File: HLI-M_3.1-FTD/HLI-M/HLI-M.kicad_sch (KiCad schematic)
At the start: 116 parts, among them CON1 , CON2 USB_B, CON3 , CON4 Connector_Adapter, CON5 Connector_Audio, CON6 Conn_01x15, CON7 Conn_01x09, CON8 CR123A, Q1 DMP3068L-7, Q2 BC817, Q3 BC817, Q4 BSS84, Q5 BSS84, Q6 BSS84, Q7 BSS84, U1 PIC24HJ64GP206-I_PT, U10 24AA02-OT, U11 ULN2003, U12 ULN2003, U13 ULN2003, U2 FM25V10-GTR, U3 MAX3232, U4 TPS7A0533PDBV, U5 TPS7A0533PDBV, U6 LM3658SD, U8 FT232RL, U9 ATSHA204A-SSHDA-B, Y1 Crystal_32KHz, Y2 Crystal_20MHz

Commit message: att
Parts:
- removed CON5: Connector_Audio, Connector_JST:JST_EH_B3B-EH-A_1x03_P2.50mm_Vertical, symbol Connector_Generic:Conn_01x03
- removed RT3: 0.5A, Resistor_SMD:R_1812_4532Metric, symbol Device:Thermistor
- added CON5: Connector_note, Connector_IDC:IDC-Header_2x04_P2.54mm_Horizontal, symbol Connector_Generic:Conn_02x04_Odd_Even
- added F1: Fuse, Fuse:Fuse_1812_4532Metric, symbol Device:Fuse
- added RV1: Varistor, Capacitor_SMD:C_0603_1608Metric_Pad1.08x0.95mm_HandSolder, symbol Device:Varistor
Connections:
- net +5V: now also CON5.1 (Pin_1), F1.2, RV1.2
- net 0: now also CON5.8 (Pin_8), RV1.1
- net INIB: now also CON5.2 (Pin_2)
- net NOTE_: now also CON5.4 (Pin_4)
- net PRINT_IMP: now also CON5.6 (Pin_6)
- net RXA: now also CON5.3 (Pin_3)
- net TXA: now also CON5.5 (Pin_5)
- net at CON1.1 (Pin_1): now also F1.1
- net EXTERN_D10: now reaches U1.44 (RD10)
- net EXTERN_D10: now also CON5.7 (Pin_7)
- no-connect marks 36 -> 35
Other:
- moved on the sheet: CON1, CON4, LED2, LED3, R25, R26, R27, R28, TP1, TP2, TP3, TP4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

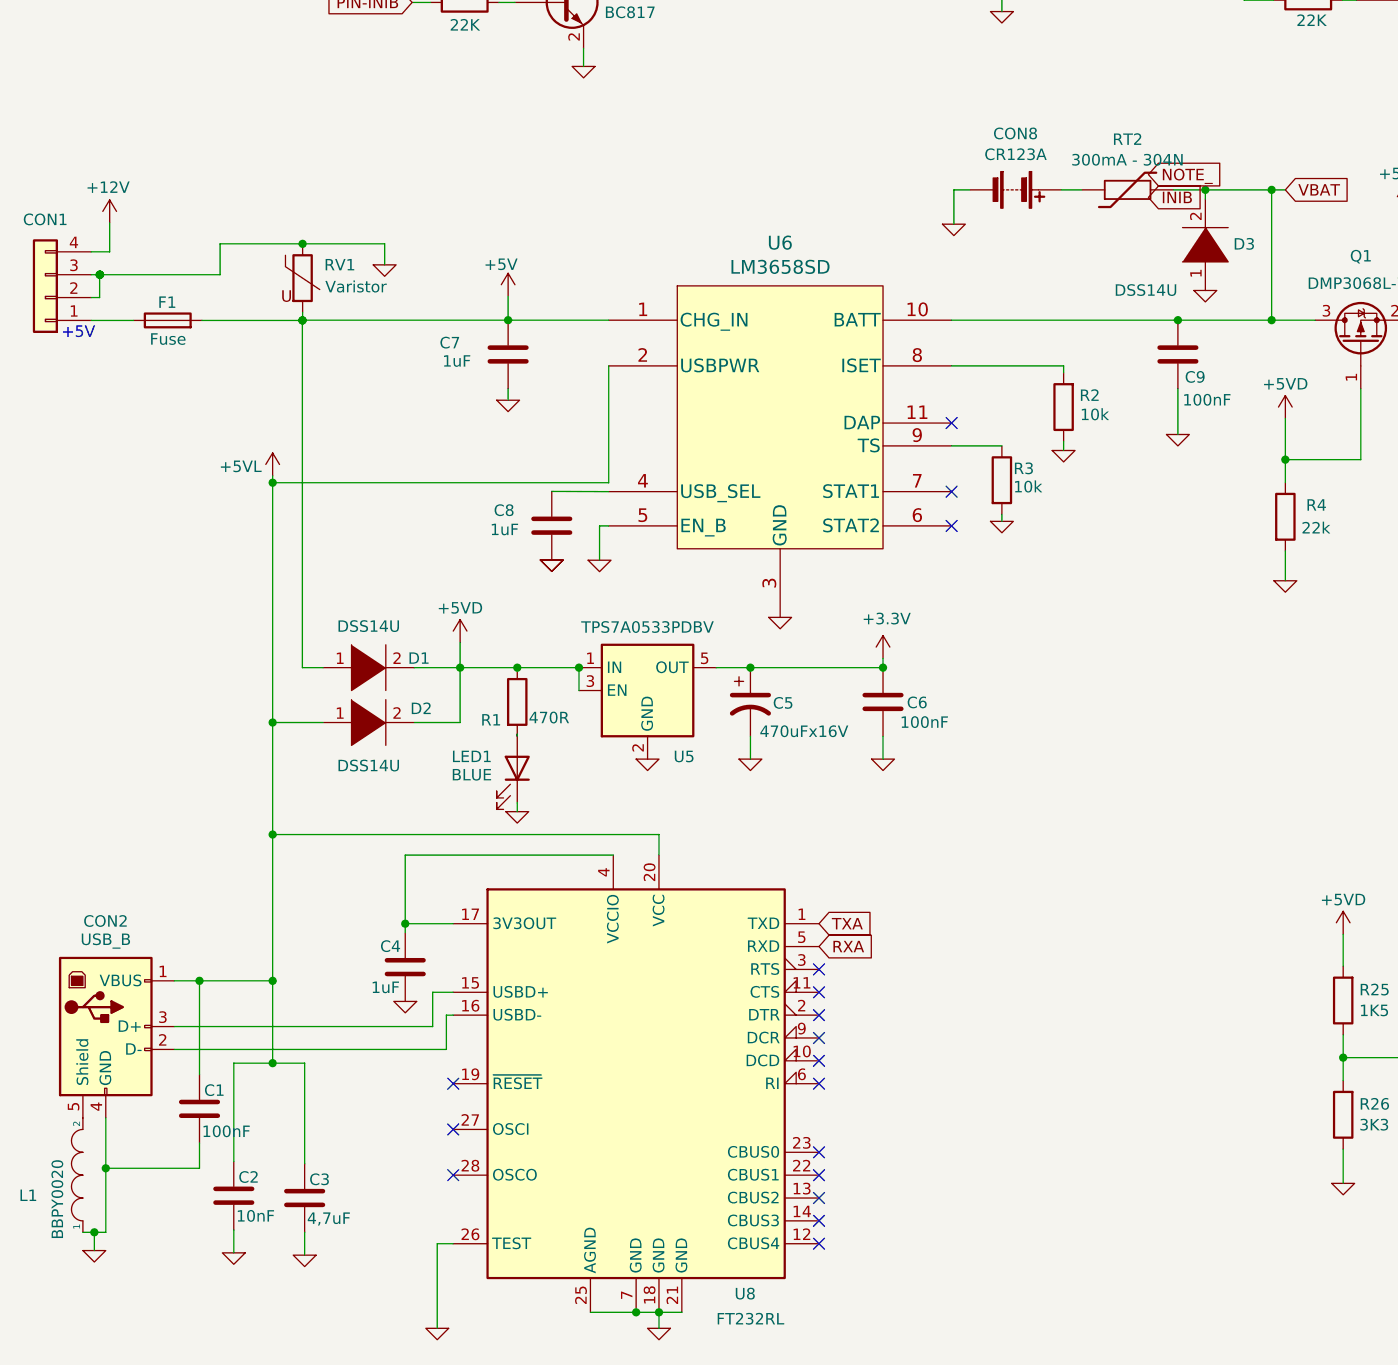
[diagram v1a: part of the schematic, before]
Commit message: att
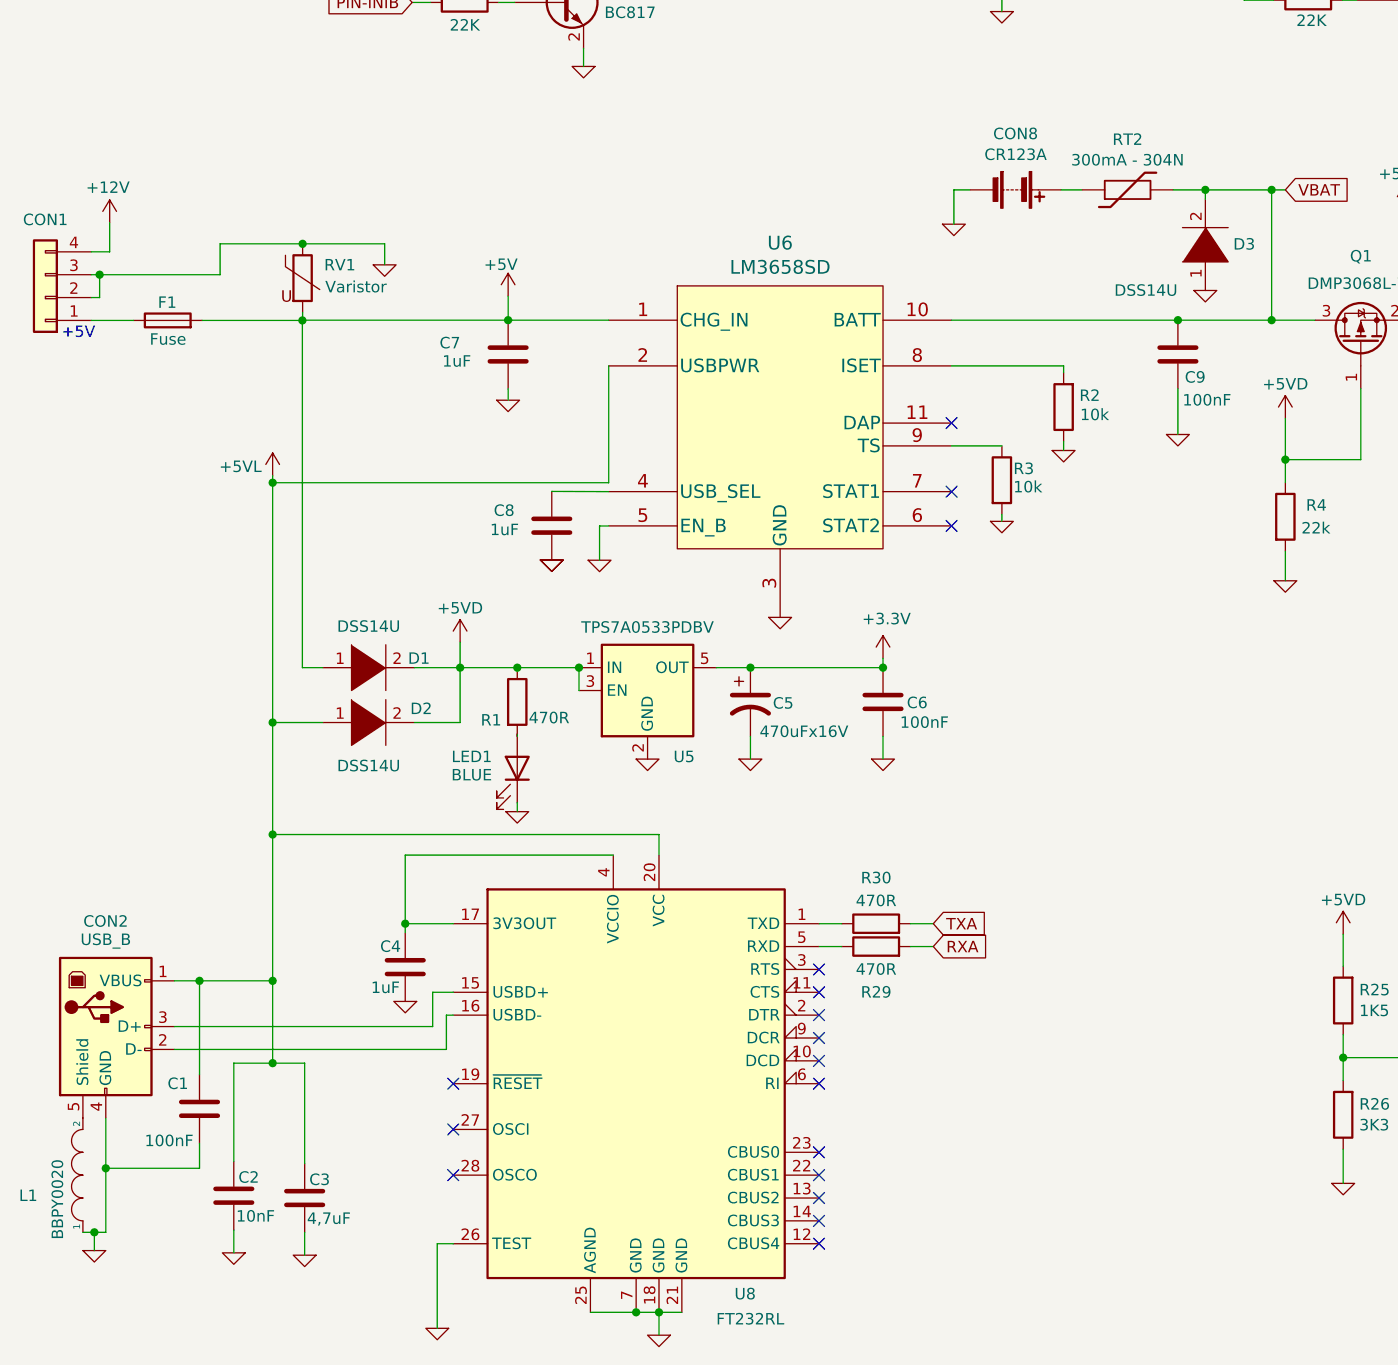
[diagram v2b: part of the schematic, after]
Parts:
- added R29, R30: 470R, symbol Device:R
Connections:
- net RXA: now also R29.2; no longer U8.5 (RXD)
- net TXA: now also R30.2; no longer U8.1 (TXD)
- new net: R29.1, U8.5 (RXD)
- new net: R30.1, U8.1 (TXD)

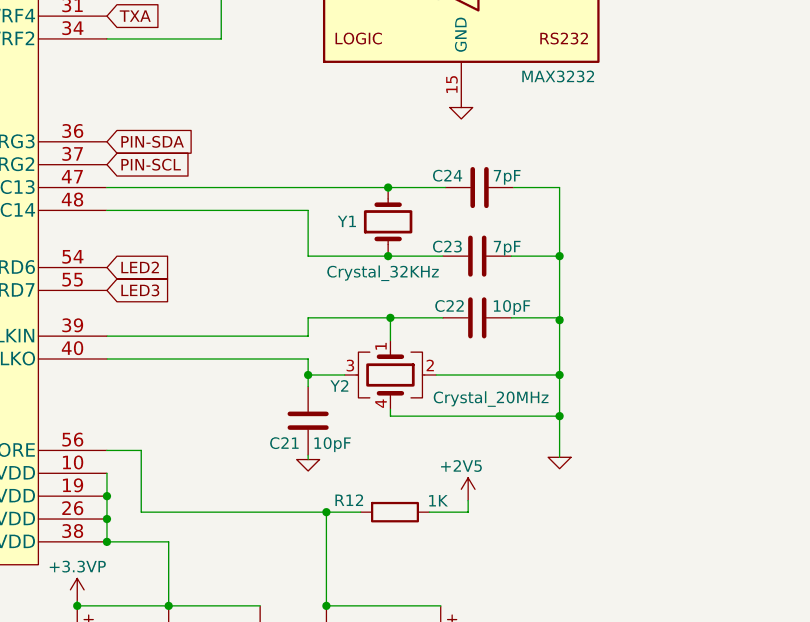
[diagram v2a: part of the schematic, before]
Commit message: atualização circuito FTD e 3D
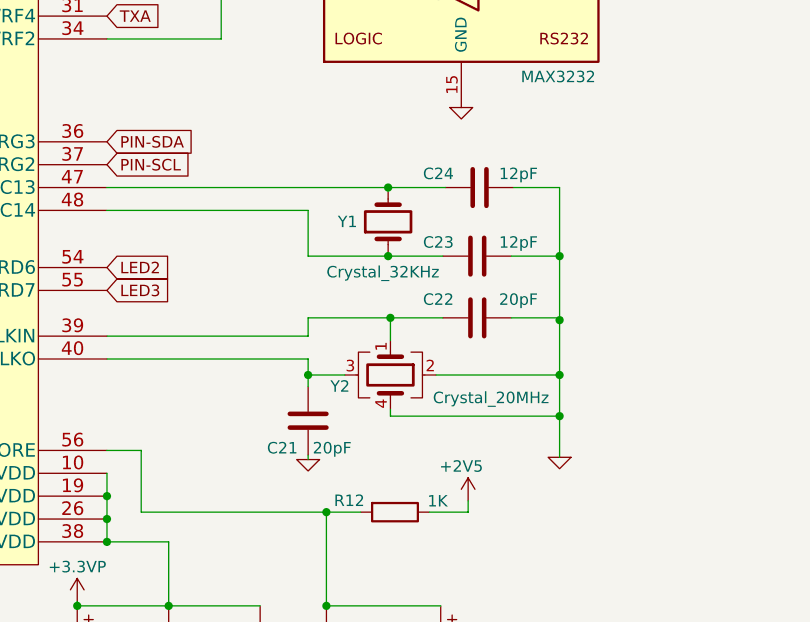
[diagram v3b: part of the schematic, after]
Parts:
- C21, C22: value 10pF -> 20pF
- C23, C24: value 7pF -> 12pF
- R29, R30: footprint (none) -> Resistor_SMD:R_0603_1608Metric_Pad0.98x0.95mm_HandSolder
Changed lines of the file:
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@@
       (effects (font (size 1.27 1.27)))
     )
-    (property "Footprint" "" (at 110.49 237.998 90)
+    (property "Footprint" "Resistor_SMD:R_0603_1608Metric_Pad0.98x0.95mm_HandSolder" (at 110.49 237.998 90)
       (effects (font (size 1.27 1.27)) hide)
     )
@@
   (symbol (lib_id "Device:C") (at 252.222 117.602 0) (unit 1)
     (in_bom yes) (on_board yes) (dnp no)
-    (property "Reference" "C21" (at 247.904 120.142 0)
-      (effects (font (size 1.27 1.27)) (justify left))
-    )
-    (property "Value" "10pF" (at 252.73 120.142 0)
+    (property "Reference" "C21" (at 247.65 120.65 0)
+      (effects (font (size 1.27 1.27)) (justify left))
+    )
+    (property "Value" "20pF" (at 252.73 120.65 0)
       (effects (font (size 1.27 1.27)) (justify left))
     )
@@
   (symbol (lib_id "Device:C") (at 271.018 106.172 90) (unit 1)
     (in_bom yes) (on_board yes) (dnp no)
-    (property "Reference" "C22" (at 267.97 104.902 90)
-      (effects (font (size 1.27 1.27)))
-    )
-    (property "Value" "10pF" (at 274.828 104.902 90)
+    (property "Reference" "C22" (at 266.7 104.14 90)
+      (effects (font (size 1.27 1.27)))
+    )
+    (property "Value" "20pF" (at 275.59 104.14 90)
       (effects (font (size 1.27 1.27)))
     )
@@
       (effects (font (size 1.27 1.27)))
     )
-    (property "Footprint" "" (at 110.49 235.458 90)
+    (property "Footprint" "Resistor_SMD:R_0603_1608Metric_Pad0.98x0.95mm_HandSolder" (at 110.49 235.458 90)
       (effects (font (size 1.27 1.27)) hide)
     )
@@
   (symbol (lib_id "Device:C") (at 271.018 99.314 90) (mirror x) (unit 1)
     (in_bom yes) (on_board yes) (dnp no)
-    (property "Reference" "C23" (at 267.716 98.298 90)
-      (effects (font (size 1.27 1.27)))
-    )
-    (property "Value" "7pF" (at 274.32 98.298 90)
+    (property "Reference" "C23" (at 266.7 97.79 90)
+      (effects (font (size 1.27 1.27)))
+    )
+    (property "Value" "12pF" (at 275.59 97.79 90)
       (effects (font (size 1.27 1.27)))
     )
@@
   (symbol (lib_id "Device:C") (at 271.272 91.694 90) (mirror x) (unit 1)
     (in_bom yes) (on_board yes) (dnp no)
-    (property "Reference" "C24" (at 267.716 90.424 90)
-      (effects (font (size 1.27 1.27)))
-    )
-    (property "Value" "7pF" (at 274.32 90.424 90)
-      (effects (font (size 1.27 1.27)))
-    )
+    (property "Reference" "C24" (at 266.7 90.17 90)
+      (effects (font (size 1.27 1.27)))
+    )
+    (property "Value" "12pF" (at 275.59 90.17 90)
+      (effects (font (size 1.27 1.27)))
+    )

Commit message: HLI-M_2023: circuito atualizado e revisado.
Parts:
- removed D1, D2, D3, D4, D5: DSS14U, Diode_SMD:D_SOD-123, symbol pspice:DIODE
- added D1, D2, D4, D5: DSS14U, Diode_SMD:D_SOD-123, symbol Device:D
- added D3: DSS14U, Diode_SMD:D_2010_5025Metric, symbol Device:D
- CON1: footprint 6:Molex-0015244449-0 -> Footprint_HLI-M:Molex-0015244449-0
- CON4: value Connector_Adapter -> Con_ADAPTER
- CON5: value Connector_note -> Con_MULTLINKER
- Q4, Q5, Q6, Q7: value BSS84 -> DMP2305
- R4: renamed from R2; value 10k -> 3,3K
- U1: value PIC24HJ64GP206-I_PT -> PIC24HJ64GP206; footprint 3:PIC24HJ64GP206-I&slash_PT -> Package_QFP:TQFP-64_10x10mm_P0.5mm
- U2: value FM25V10-GTR -> FM25V10; footprint 4:FM25V10-GTR -> Footprint_HLI-M:FM25V10-GTR
- U4: renamed from U9; footprint 1:ATSHA204A-SSHDA-B -> Package_SO:SOIC-8_3.9x4.9mm_P1.27mm
- U6: footprint 2:LM3658SD -> Footprint_HLI-M:LM3658SD
- renumbered C24 to C23, C23 to C24, R30 to R1, R8 to R10, R9 to R11, R10 to R12, R11 to R13, R12 to R14, R13 to R15, R14 to R16, R15 to R17, R16 to R18, R17 to R19, R29 to R2, R18 to R20, R19 to R21, R20 to R22, R21 to R23, R22 to R24, R23 to R25, R24 to R26, R25 to R29, R1 to R3, R26 to R30, R3 to R5, R4 to R6, R5 to R7, R6 to R8, R7 to R9, U11 to U10, U12 to U11, U13 to U12, U10 to U5, U4 to U7, U5 to U8, U8 to U9
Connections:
- net +5V: now also D1.2 (A), D4.2 (A)
- net +5VD: now also D1.1 (K), D2.1 (K)
- net +5VL: now also D2.2 (A), D5.2 (A)
- net 0: now also U6.11 (DAP), D3.2 (A)
- net CIN: now also CON6.12 (Pin_12), Q7.3 (D); no longer CON6.13 (Pin_13), Q6.3 (D)
- net COUT: now also CON6.13 (Pin_13), Q6.3 (D); no longer CON6.12 (Pin_12), Q7.3 (D)
- net PGEC2: now also R10.1; no longer R11.1
- net PGED2: now also R11.1; no longer R10.1
- net PIN-CIN: now also R11.2, U12.1 (I1); no longer R10.2, U12.2 (I2)
- net PIN-COUT: now also R10.2, U12.2 (I2); no longer R11.2, U12.1 (I1)
- net VBAT: now also D3.1 (K)
- net at C10.1, C11.1, Q1.2 (S)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: now also D4.1 (K), D5.1 (K)
- net at C23.1, Y1.2: now also U1.48 (RC14); no longer U1.47 (RC13)
- net at C24.1, Y1.1: now also U1.47 (RC13); no longer U1.48 (RC14)
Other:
- note added: "ALIMENTAÇÃO E COMUNICAÇÃO USB."
- note added: "CHIP ENCRIPTAÇÃO."
- note added: "CONECTORES PARA BOTÕES, GRAVAÇÃO E MULTLINKER."
- note added: "EEPROM."
- note added: "IMPRESSORA E NOTEIRO."
- note added: "LEDS LOCKBITS."
- note added: "LÂMPADAS E CONTADORES."
- note added: "PONTOS DE TESTE."
- note added: "PROCESSADOR, FRAM E COMUNICAÇÃO SERIAL."
- company: (none) -> ORION GAMES.
- title: (none) -> HLI-M 2023 PROJECT. 
- moved on the sheet: C1, C10, C11, C12, C13, C14, C15, C16, C17, C18, C19, C2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

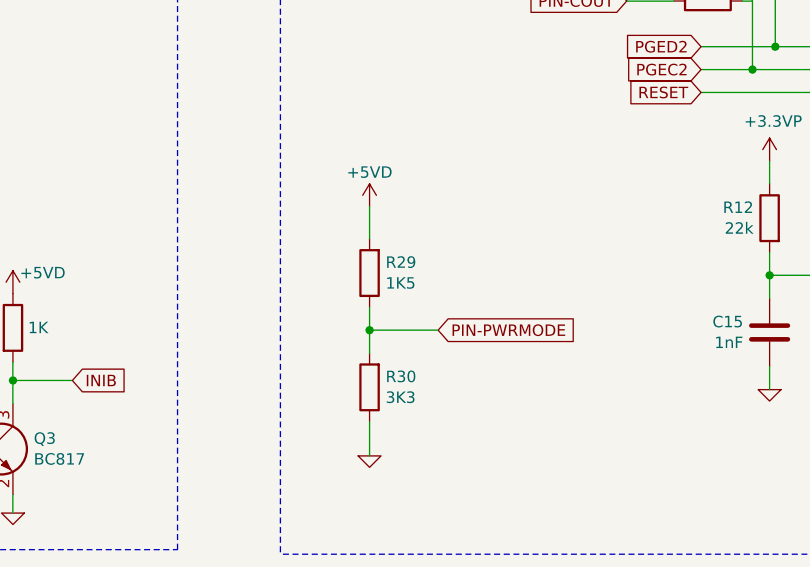
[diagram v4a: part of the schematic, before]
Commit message: HLI-C 2023: atualizado e revisado.
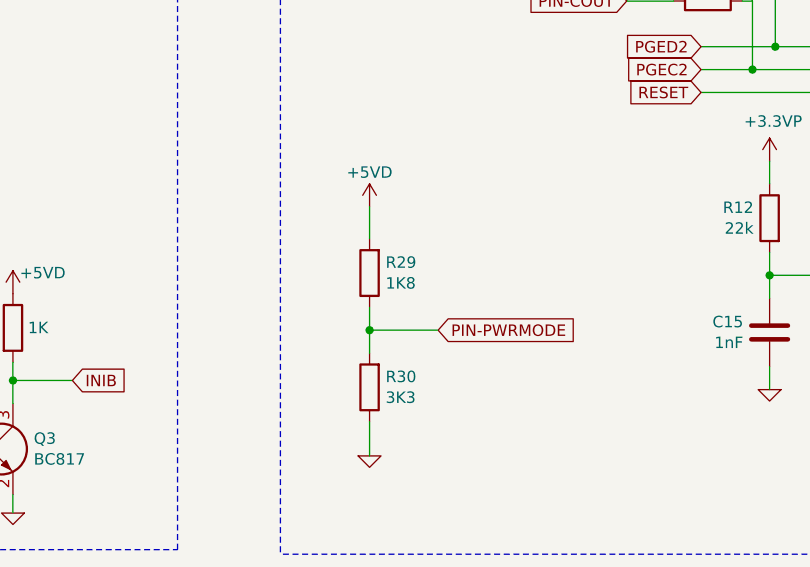
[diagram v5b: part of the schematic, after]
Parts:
- R29: value 1K5 -> 1K8
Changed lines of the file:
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@@
       (effects (font (size 1.27 1.27)) (justify right))
     )
-    (property "Value" "1K5" (at 119.126 132.969 0)
+    (property "Value" "1K8" (at 119.126 132.969 0)
       (effects (font (size 1.27 1.27)) (justify right))
     )
